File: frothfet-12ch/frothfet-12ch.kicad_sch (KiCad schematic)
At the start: 8 parts

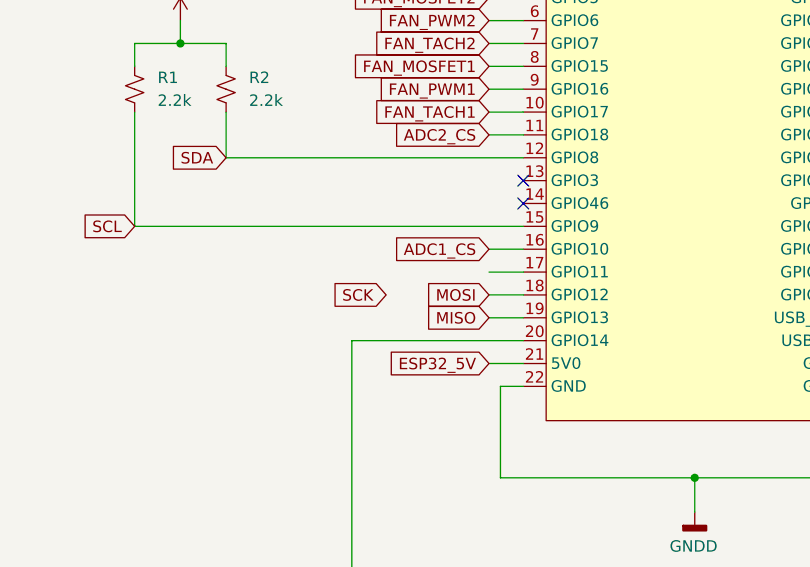
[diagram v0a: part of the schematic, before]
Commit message: clean drc
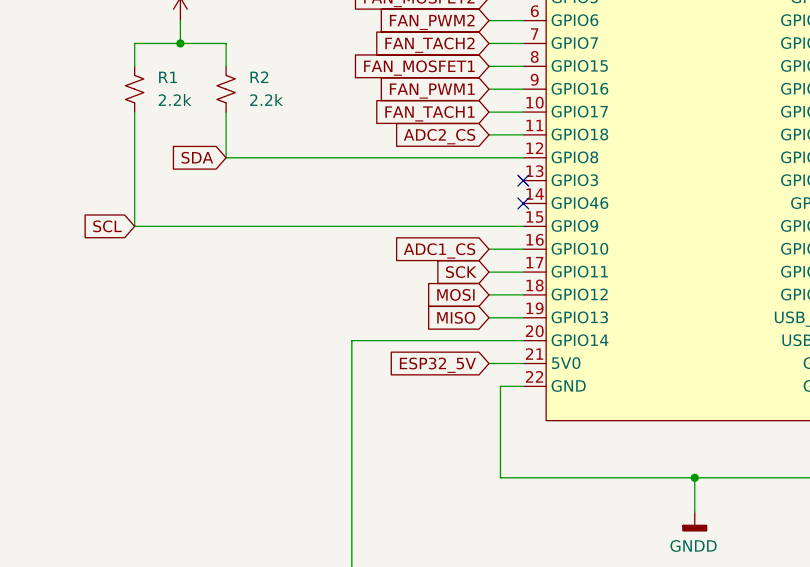
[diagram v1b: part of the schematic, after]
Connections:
- net SCK: now also U1.17 (GPIO11)
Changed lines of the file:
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@@
 	(global_label "SCK"
 		(shape input)
-		(at 105.41 102.87 180)
+		(at 116.84 100.33 180)
 		(fields_autoplaced yes)
 		(effects
@@
 		)
 		(property "Intersheetrefs" "${INTERSHEET_REFS}"
-			(at 98.6753 102.87 0)
+			(at 110.1053 100.33 0)
 			(effects
 				(font
